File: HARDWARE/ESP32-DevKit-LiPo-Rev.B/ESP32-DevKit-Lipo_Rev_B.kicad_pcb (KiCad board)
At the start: 2 copper layers, 27.9 x 48.3 mm, 58 parts, among them Q1 Q12MHz/20pF/10ppm/4P/3.2x2.5mm, Q2 BC817-40(SOT23), Q3 BC817-40(SOT23), U1 BL4054B-42TPRN(SOT23-5), U2 CH340T(SSOP20W), U3 SY8089AAAC(SOT23-5), U5 ESP32-WROOM-32D-4MB

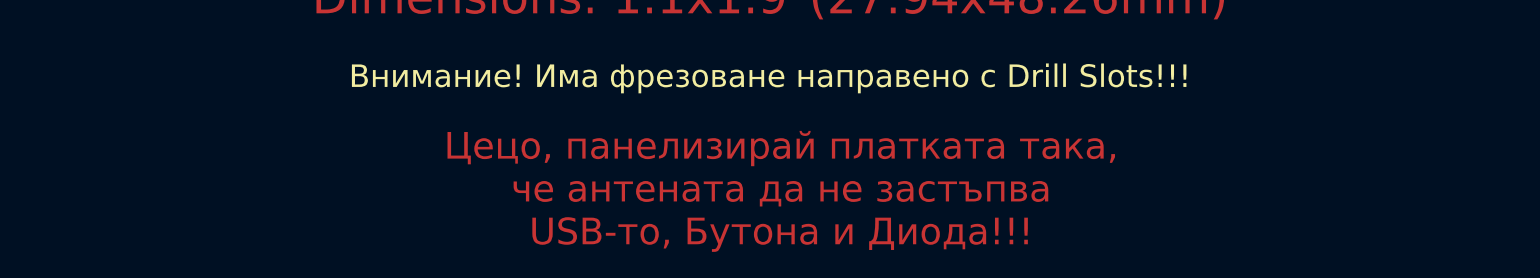
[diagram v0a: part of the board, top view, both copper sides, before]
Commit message: Update
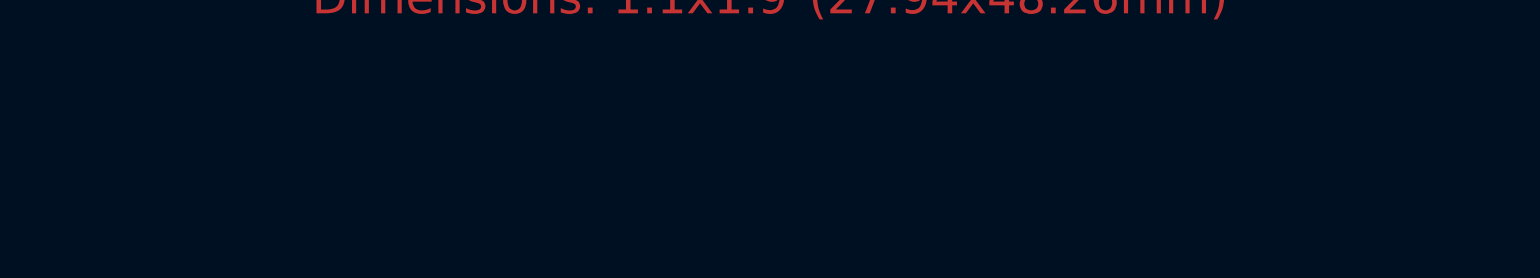
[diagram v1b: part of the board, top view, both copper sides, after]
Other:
- board text removed: "Цецо, панелизирай платката така, че антената да не застъпва USB-то, Бутона и Диода!!!"
